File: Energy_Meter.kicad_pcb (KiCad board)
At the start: 2 copper layers, 74.9 x 87.6 mm, 78 parts, among them CON1 Fuente, IC1 Corriente C, J5 TENSION, J6 PROGRAMACION, Q1 BC817, Q2 BC817, SW1 RESET, SW2 PROG, U1 ESP32-WROOM-32D, U2 ATM90E36, U3 LD1117S18TR_SOT223, Y1 16.384MHz

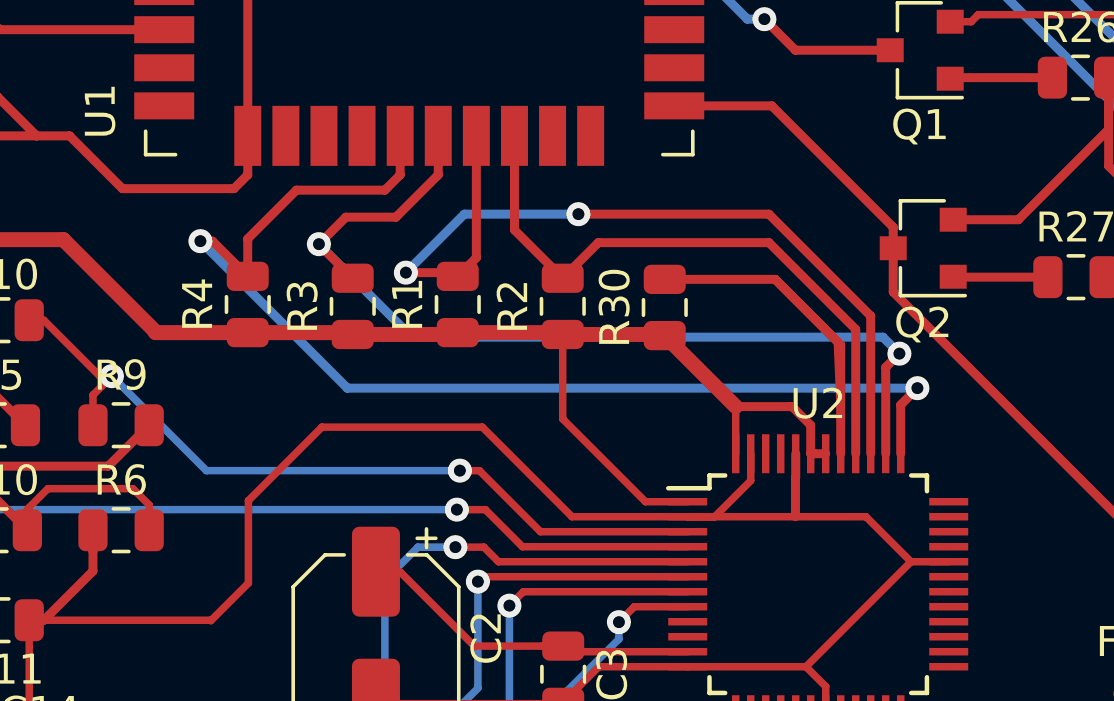
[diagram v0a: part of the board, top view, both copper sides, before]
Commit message: Add files via upload
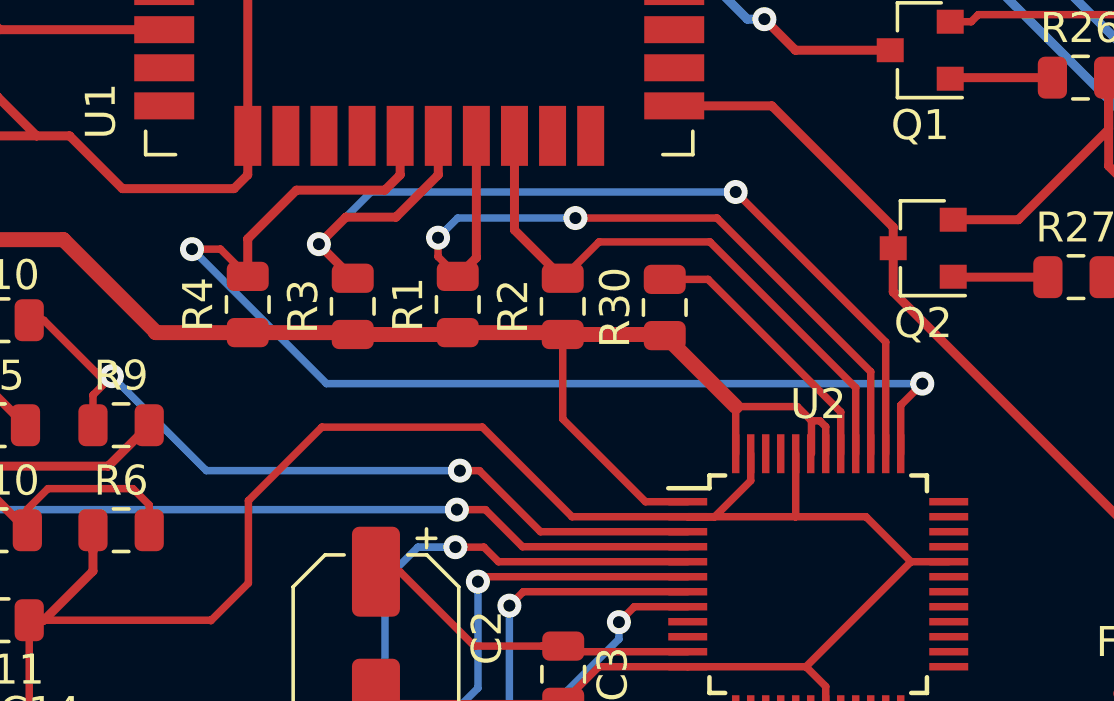
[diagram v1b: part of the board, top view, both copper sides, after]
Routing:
- net Net-(R30-Pad2): track 17.1 -> 9.09 mm
- net /MISO: track 29.0 -> 26.0 mm
- net /MOSI: track 21.0 -> 19.9 mm
- net +3V3: track 208.7 -> 209.7 mm
- net /CLK: track 32.2 -> 33.2 mm
- net /CS: track 38.9 -> 39.6 mm
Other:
- net class Default: clearance 0.1524 -> 0.25
- rule trace_clearance: 0.1524 -> 0.25
